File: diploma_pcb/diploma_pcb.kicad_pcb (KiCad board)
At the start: 2 copper layers, 50 x 24 mm, 17 parts, among them Q1 2SC3356, Q3 2SC3356

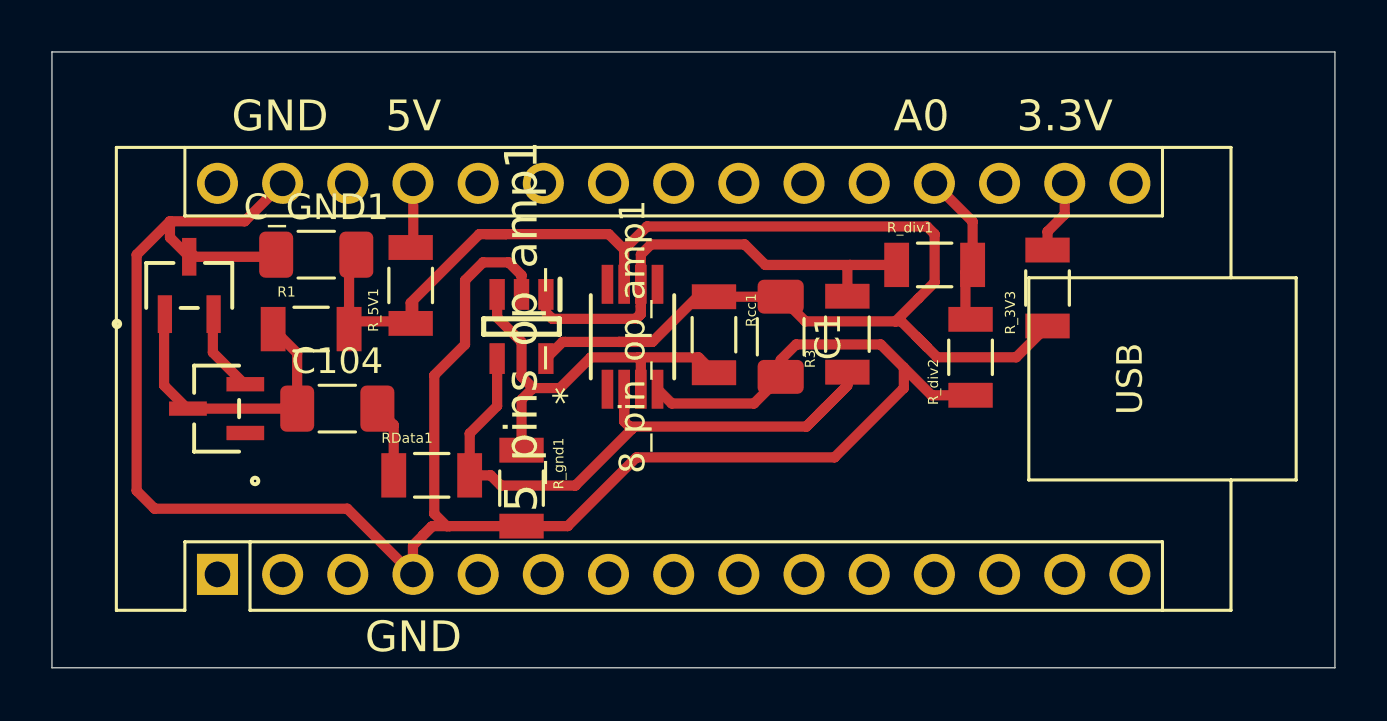
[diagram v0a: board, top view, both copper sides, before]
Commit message: rgb placed
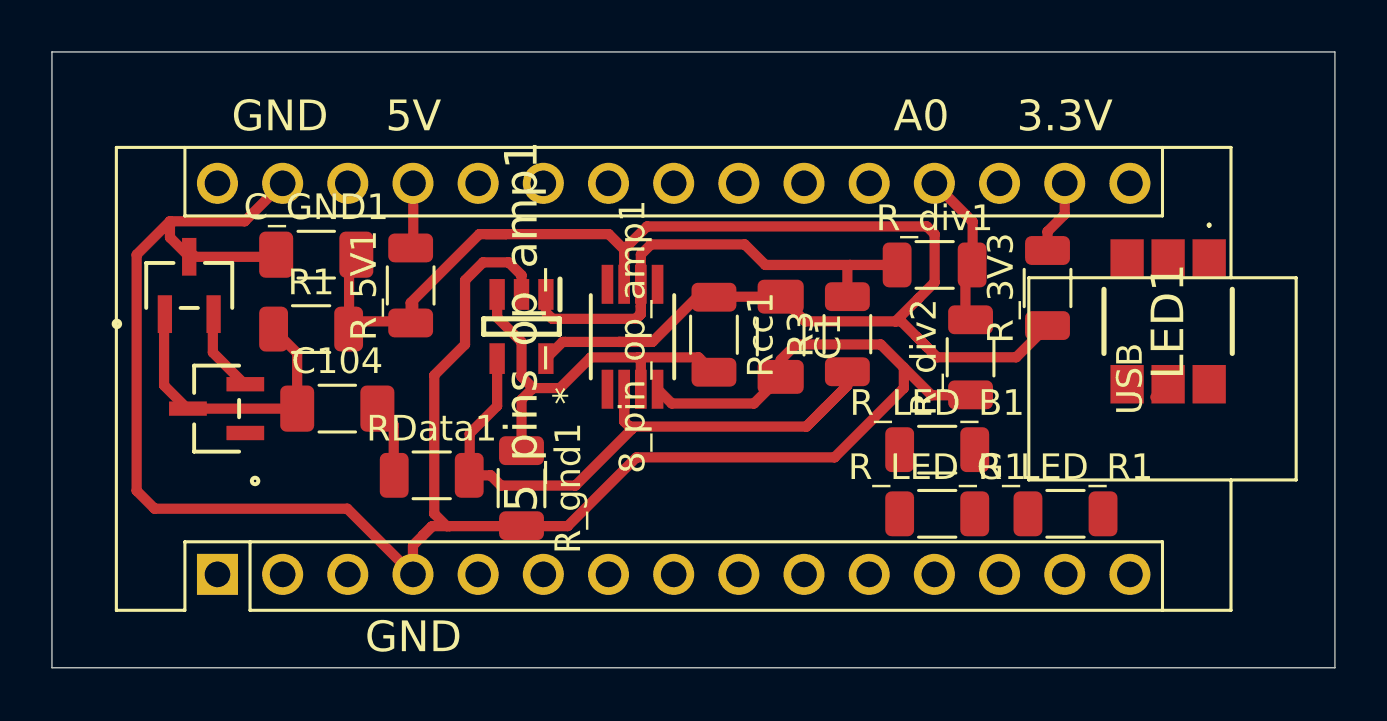
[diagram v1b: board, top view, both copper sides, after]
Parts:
- added LED1: MP008253, MP008253:MP008253, F.Cu at (69.5, 60.0)
- added R_LED_B1: R, Resistor_SMD:R_1206_3216Metric, F.Cu at (60.5, 65.0)
- added R_LED_G1: R, Resistor_SMD:R_1206_3216Metric, F.Cu at (60.5, 67.5)
- added R_LED_R1: R, Resistor_SMD:R_1206_3216Metric, F.Cu at (65.5, 67.5)
- R1, R3, RData1, R_3V3, R_5V1, R_div1, R_div2, R_gnd1, Rcc1: footprint 1206:RESC3116X65N -> Resistor_SMD:R_1206_3216Metric
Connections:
- A1 pad 11: unconnected-(A1-D8-Pad11) -> Net-(A1-D8)
- A1 pad 12: unconnected-(A1-D9-Pad12) -> Net-(A1-D9)
- A1 pad 13: unconnected-(A1-D10-Pad13) -> Net-(A1-D10)
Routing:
- net Net-(LED1-A_GREEN): track 0.00 -> 0.71 mm
- net Net-(LED1-A_RED): track 0.00 -> 0.57 mm

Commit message: Working Serial Comunication!
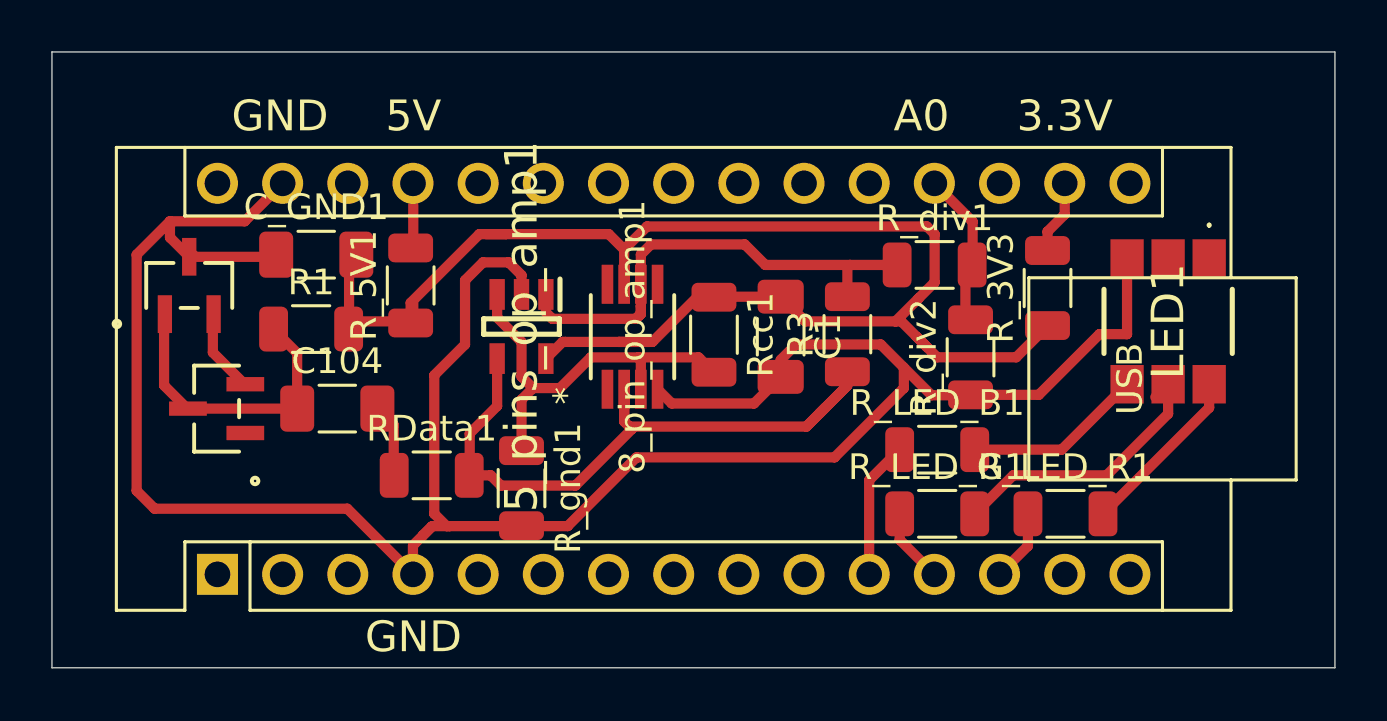
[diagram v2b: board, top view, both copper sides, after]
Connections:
- net Net-(5_pins_op_amp1-VIN+) renamed non inv
- net Net-(5_pins_op_amp1-VOUT) renamed Vout
- net Net-(A1-+5V) renamed 5V
- net Net-(A1-3V3) renamed 3.3V
- net Net-(LED1-A_BLUE) renamed blue
- net Net-(LED1-A_GREEN) renamed green
- net Net-(LED1-A_RED) renamed red
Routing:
- net green: track 0.71 -> 11.0 mm
- net GND: track 86.1 -> 96.1 mm
- net blue: track 0.00 -> 6.99 mm
- net red: track 0.57 -> 7.33 mm
- net Net-(A1-D8): track 0.00 -> 5.35 mm
- net Net-(A1-D9): track 0.00 -> 2.92 mm
- net Net-(A1-D10): track 0.00 -> 2.82 mm
